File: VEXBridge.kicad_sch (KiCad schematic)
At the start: 28 parts, among them J1 4P4C, J3 Conn_01x05_Pin, U1 LM2596S-5, U2 MAX481E, U5 SN74LVC2G14DBV

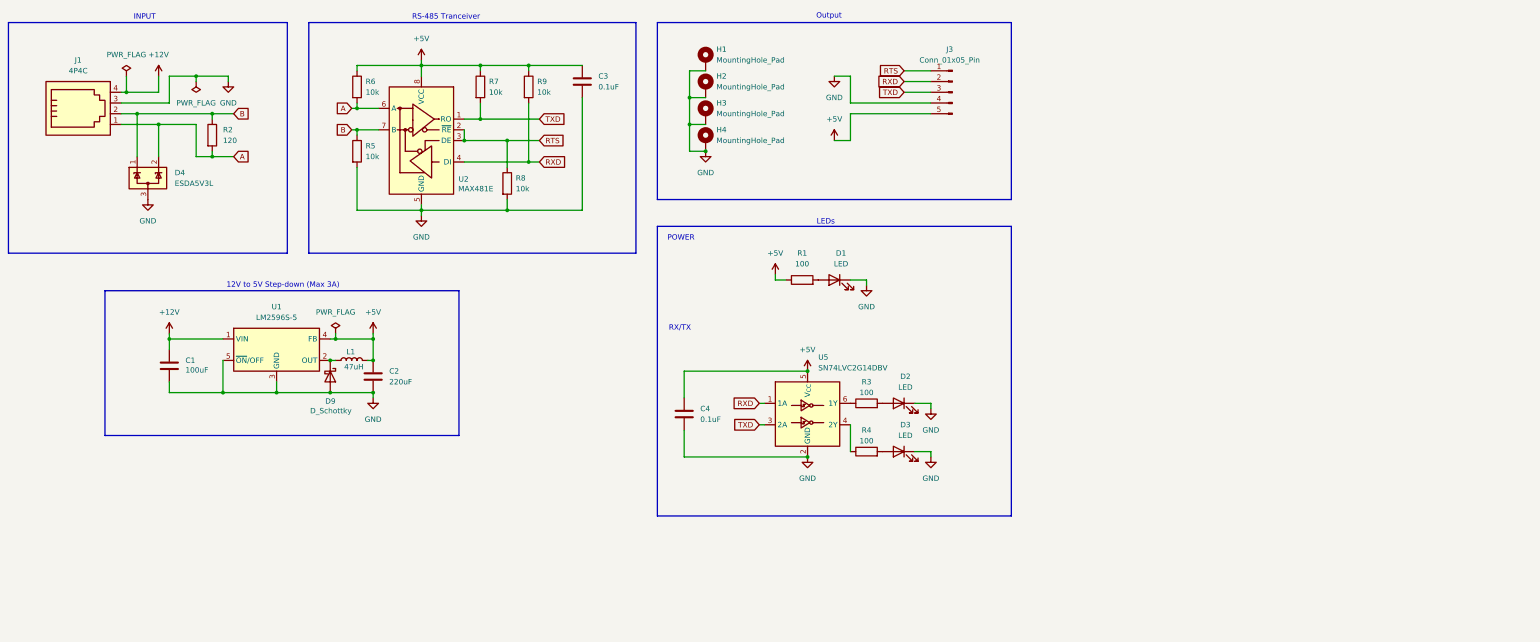
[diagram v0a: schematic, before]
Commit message: VEXBridge v2 (WIP)
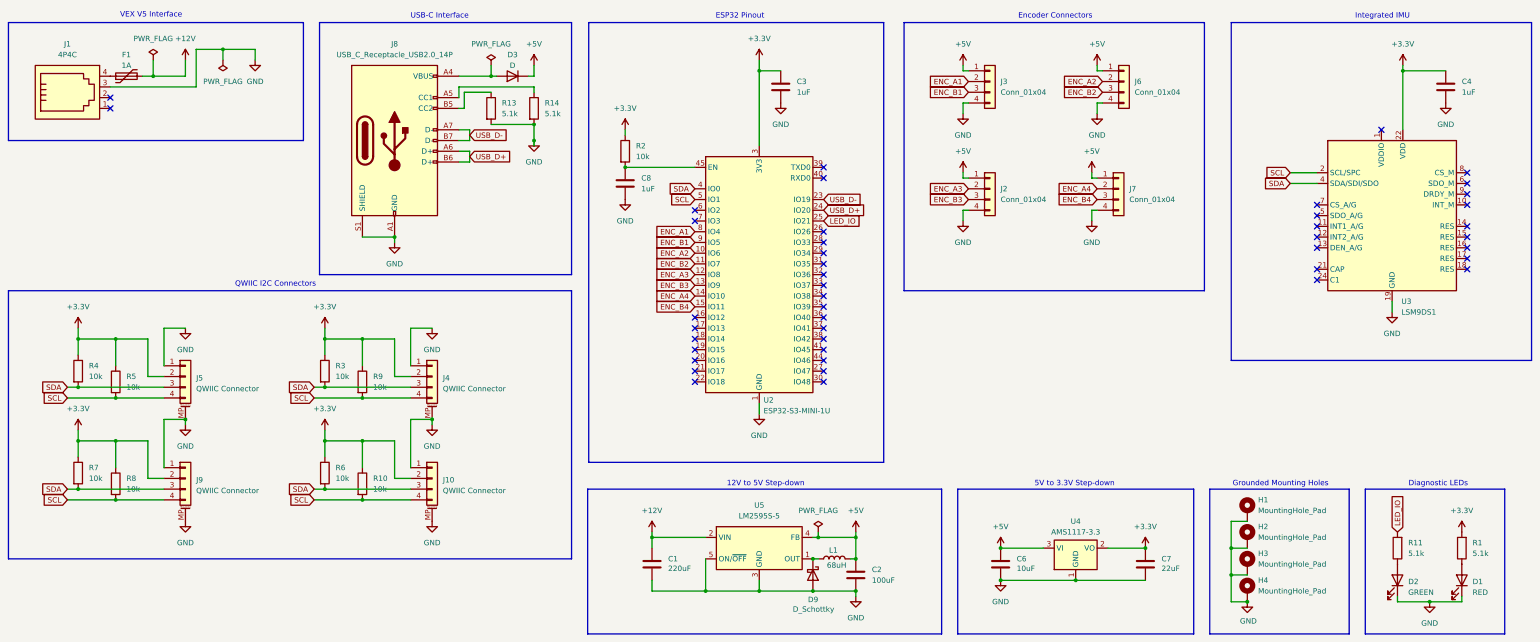
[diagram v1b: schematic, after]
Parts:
- removed D3: LED, LED_SMD:LED_0603_1608Metric, symbol Device:LED
- removed D4: ESDA5V3L, Package_TO_SOT_SMD:SOT-23-3, symbol Power_Protection:ESDA5V3L
- removed J3: Conn_01x05_Pin, Connector_PinHeader_2.54mm:PinHeader_1x05_P2.54mm_Vertical, symbol Connector:Conn_01x05_Pin
- removed U1: LM2596S-5, Package_TO_SOT_SMD:TO-263-5_TabPin3, symbol Regulator_Switching:LM2596S-5
- removed U2: MAX481E, Package_SO:SOIC-8_3.9x4.9mm_P1.27mm, symbol Interface_UART:MAX481E
- removed U5: SN74LVC2G14DBV, Package_TO_SOT_SMD:SOT-23-6, symbol 74xGxx:SN74LVC2G14DBV
- added C6: 10uF, Capacitor_SMD:C_0201_0603Metric, symbol Device:C
- added C7: 22uF, Capacitor_SMD:C_1206_3216Metric, symbol Device:C
- added C8: 1uF, Capacitor_SMD:C_0201_0603Metric, symbol Device:C
- added D3: D, Diode_SMD:D_0201_0603Metric, symbol Device:D
- added F1: 1A, Fuse:Fuse_2010_5025Metric, symbol Device:Polyfuse
- added J10, J4, J5, J9: QWIIC Connector, Connector_JST:JST_SH_SM04B-SRSS-TB_1x04-1MP_P1.00mm_Horizontal, symbol Connector_Generic_MountingPin:Conn_01x04_MountingPin
- added J2, J3, J6, J7: Conn_01x04, Connector_Molex:Molex_PicoBlade_53047-0410_1x04_P1.25mm_Vertical, symbol Connector_Generic:Conn_01x04
- added J8: USB_C_Receptacle_USB2.0_14P, Connector_USB:USB_C_Plug_Molex_105444, symbol Connector:USB_C_Receptacle_USB2.0_14P
- added R10: 10k, Resistor_SMD:R_0805_2012Metric, symbol Device:R
- added R11, R13, R14: 5.1k, Resistor_SMD:R_0805_2012Metric, symbol Device:R
- added U2: ESP32-S3-MINI-1U, RF_Module:ESP32-S2-MINI-1U, symbol RF_Module:ESP32-S3-MINI-1U
- added U3: LSM9DS1, Package_LGA:LGA-24L_3x3.5mm_P0.43mm, symbol Sensor_Motion:LSM9DS1
- added U4: AMS1117-3.3, Package_TO_SOT_SMD:SOT-223-3_TabPin2, symbol Regulator_Linear:AMS1117-3.3
- added U5: LM2595S-5, Package_TO_SOT_SMD:TO-263-5_TabPin3, symbol Regulator_Switching:LM2595S-5
- C1: value 100uF -> 220uF; footprint Capacitor_SMD:CP_Elec_6.3x7.7 -> Capacitor_SMD:C_1210_3225Metric
- C2: value 220uF -> 100uF; footprint Capacitor_SMD:CP_Elec_6.3x7.7 -> Capacitor_SMD:C_1206_3216Metric
- C3, C4: value 0.1uF -> 1uF; footprint Capacitor_SMD:C_0402_1005Metric -> Capacitor_SMD:C_0201_0603Metric
- D1: value LED -> RED
- D2: value LED -> GREEN
- L1: value 47uH -> 68uH; footprint Inductor_SMD:L_Coilcraft_LPS4018 -> Inductor_SMD:L_SXN_SMDRI127
- R1: value 100 -> 5.1k
- R2: value 120 -> 10k; footprint Resistor_SMD:R_1206_3216Metric -> Resistor_SMD:R_0805_2012Metric
- R3, R4: value 100 -> 10k
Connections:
- net RTS is gone; now on net +3.3V: R8.1
- net TXD is gone; now on net SDA: R7.2
- net +12V: now also F1.2, U5.2 (VIN); no longer J1.4
- net +5V: now also C6.1, D3.1 (K), J2.1 (Pin_1), J3.1 (Pin_1), J6.1 (Pin_1), J7.1 (Pin_1), U4.3 (VI), U5.4 (FB); no longer C3.1, C4.1, R1.1, R6.1, R7.1, R9.1
- net GND: now also C6.2, C7.2, C8.2, J10.1 (Pin_1), J10.MP (MountPin), J2.4 (Pin_4), J3.4 (Pin_4), J4.1 (Pin_1), J4.MP (MountPin), J5.1 (Pin_1), J5.MP (MountPin), J6.4 (Pin_4), J7.4 (Pin_4), J8.A1 (GND), J8.A12 (GND), J8.B1 (GND), J8.B12 (GND), J8.S1 (SHIELD), J9.1 (Pin_1), J9.MP (MountPin), R13.2, R14.2, U2.1 (GND), U2.2 (GND), U2.42 (GND), U2.43 (GND), U2.46 (GND), U2.47 (GND), U2.48 (GND), U2.49 (GND), U2.50 (GND), U2.51 (GND), U2.52 (GND), U2.53 (GND), U2.54 (GND), U2.55 (GND), U2.56 (GND), U2.57 (GND), U2.58 (GND), U2.59 (GND), U2.60 (GND), U2.61 (GND), U2.62 (GND), U2.63 (GND), U2.64 (GND), U2.65 (GND), U3.19 (GND), U3.20 (GND), U4.1 (GND), U5.3 (GND), U5.5 (ON/~{OFF}); no longer R5.2, R8.2
- net +3.3V: now reaches R4.1
- net +3.3V: now also C3.1, C4.1, R1.2, R2.1, R3.1, R5.1, R6.1, R7.1, R9.1, C7.1, J10.2 (Pin_2), J4.2 (Pin_2), J5.2 (Pin_2), J9.2 (Pin_2), R10.1, U2.3 (3V3), U3.22 (VDD), U3.23 (VDD), U4.2 (VO)
- net SDA: now reaches R4.2
- net SDA: now also R3.2, R6.2, J10.3 (Pin_3), J4.3 (Pin_3), J5.3 (Pin_3), J9.3 (Pin_3), U2.4 (IO0), U3.4 (SDA/SDI/SDO)
- net at D9.1 (K), L1.1: now also U5.1 (OUT)
- net at D1.2 (A): now also R1.1; no longer R1.2
- net at D2.2 (A): now also R11.1; no longer R3.2
- removed net A: J1.1, R2.2, R6.2
- removed net B: J1.2, R2.1, R5.1
- net RXD renamed SCL
- net SCL: now also R5.2, R8.2, J10.4 (Pin_4), J4.4 (Pin_4), J5.4 (Pin_4), J9.4 (Pin_4), R10.2, U2.5 (IO1), U3.2 (SCL/SPC)
- new net: F1.1, J1.4
- new net: C8.1, R2.2, U2.45 (EN)
- new net: U3.1 (VDDIO), U3.3 (VDDIO)
- new net: J8.B5 (CC2), R13.1
- new net: J8.A5 (CC1), R14.1
- new net: D3.2 (A), J8.A4 (VBUS), J8.A9 (VBUS), J8.B4 (VBUS), J8.B9 (VBUS)
- new net ENC_A1: J3.2 (Pin_2), U2.8 (IO4)
- new net ENC_A2: J6.2 (Pin_2), U2.10 (IO6)
- new net ENC_A3: J2.2 (Pin_2), U2.12 (IO8)
- new net ENC_A4: J7.2 (Pin_2), U2.14 (IO10)
- new net ENC_B1: J3.3 (Pin_3), U2.9 (IO5)
- new net ENC_B2: J6.3 (Pin_3), U2.11 (IO7)
- new net ENC_B3: J2.3 (Pin_3), U2.13 (IO9)
- new net ENC_B4: J7.3 (Pin_3), U2.15 (IO11)
- new net LED_IO: R11.2, U2.25 (IO21)
- new net USB_D+: J8.A6 (D+), J8.B6 (D+), U2.24 (IO20)
- new net USB_D-: J8.A7 (D-), J8.B7 (D-), U2.23 (IO19)
- no-connect marks 0 -> 45
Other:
- note added: "12V to 5V Step-down"
- note added: "5V to 3.3V Step-down"
- note added: "Diagnostic LEDs"
- note added: "ESP32 Pinout"
- note added: "Encoder Connectors"
- note added: "Grounded Mounting Holes"
- note added: "Integrated IMU"
- note added: "QWIIC I2C Connectors"
- note added: "USB-C Interface"
- note added: "VEX V5 Interface"
- note removed: "12V to 5V Step-down (Max 3A)"
- note removed: "INPUT"
- note removed: "LEDs"
- note removed: "Output"
- note removed: "POWER"
- note removed: "RS-485 Tranceiver"
- note removed: "RX/TX"
- moved on the sheet: C1, C2, D1, D9, H1, H2, H3, H4, J1, L1, R1
